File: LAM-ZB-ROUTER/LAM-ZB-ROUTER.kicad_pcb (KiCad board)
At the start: 2 copper layers, 40 x 60 mm, 12 parts, among them J1 PWR, J2 Conn_01x07_Pin, U1 CC2538, U2 LT1117-3.3

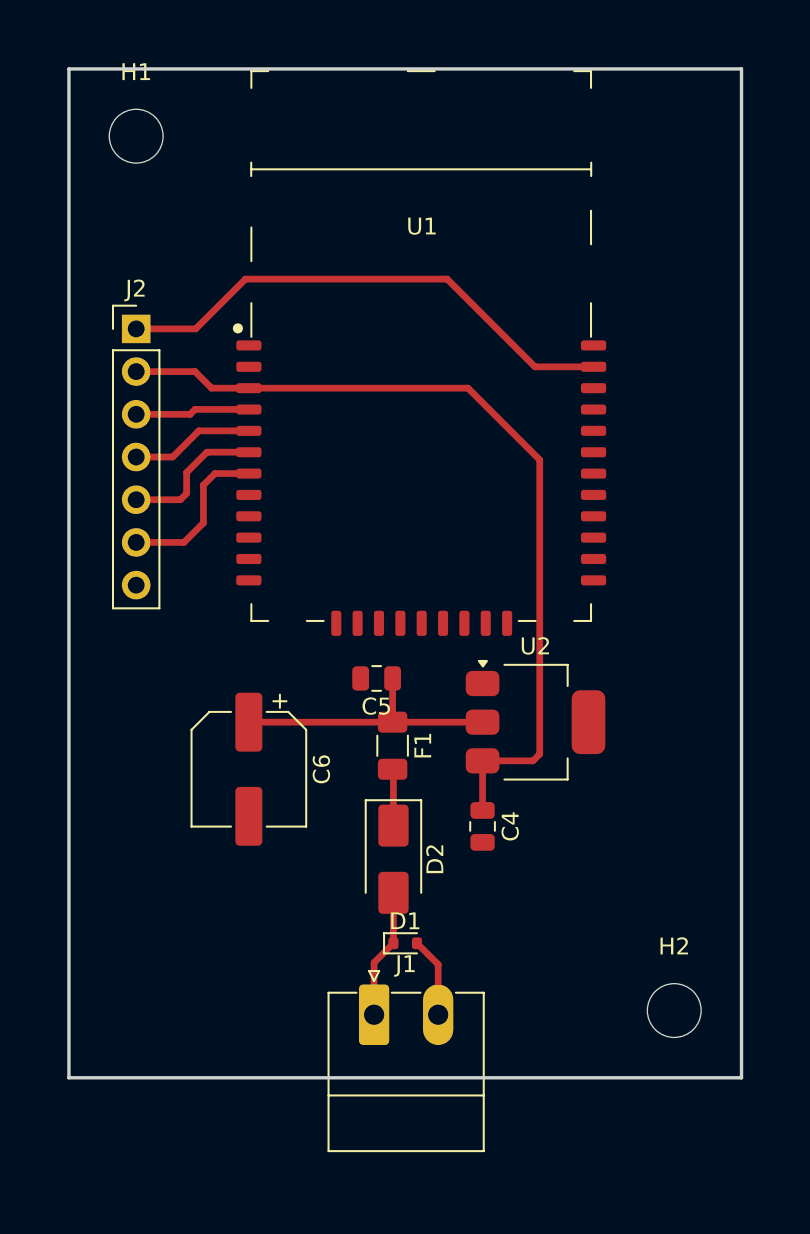
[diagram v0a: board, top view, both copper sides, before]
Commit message: LAM-ZB-ROUTER: Rev B
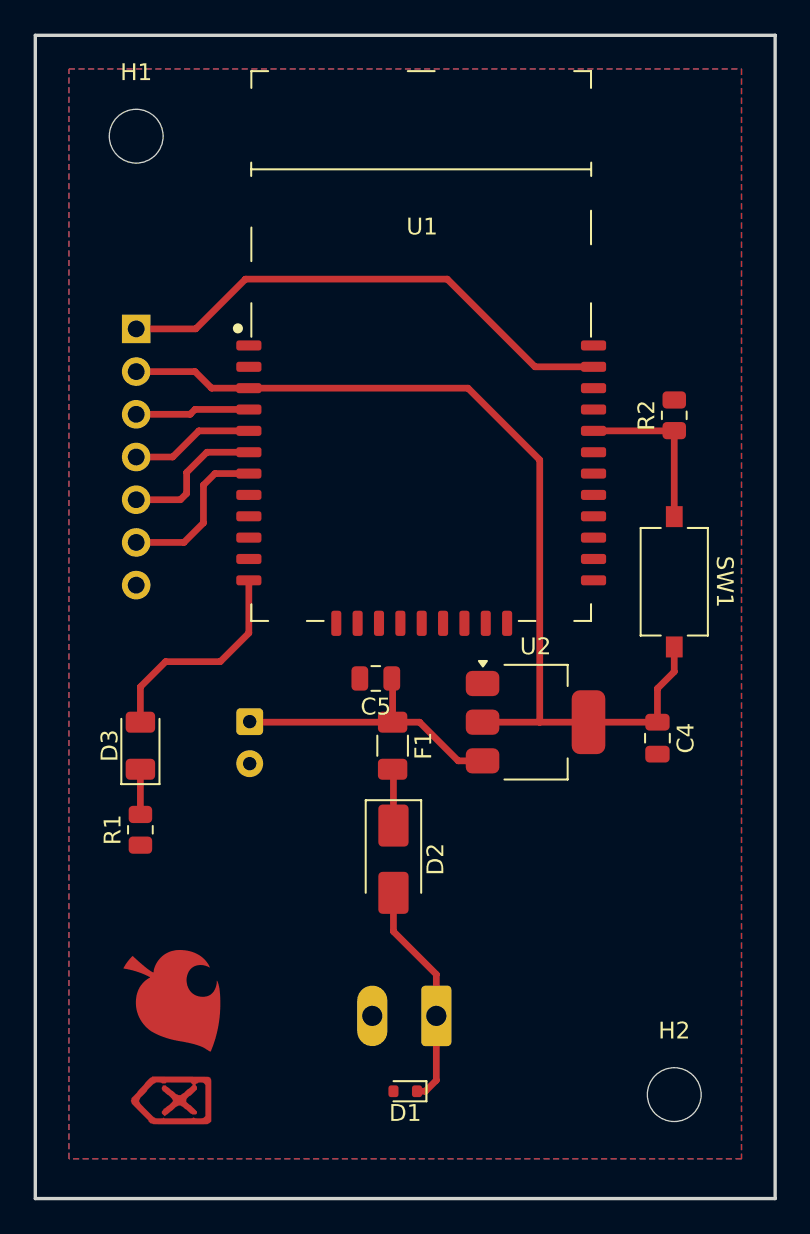
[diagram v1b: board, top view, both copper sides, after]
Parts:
- removed C6: 470uF / 25V, Capacitor_SMD:CP_Elec_6.3x5.9
- added C1: 100uF / 25V, Capacitor_THT:CP_Radial_D6.3mm_P2.50mm, B.Cu at (140.8, 108.8)
- added D3: RUN, LED_SMD:LED_1206_3216Metric, F.Cu at (134.2, 110.2)
- added R1: 270R, Resistor_SMD:R_0805_2012Metric, F.Cu at (134.2, 115.2)
- added R2: 5K1, Resistor_SMD:R_0805_2012Metric, F.Cu at (166.0, 90.6)
- added REF**: 0x08_F_Cu, Logos:0x08_F_Cu, F.Cu at (136.1, 131.3)
- added SW1: FLASH, Button_Switch_SMD:SW_Tactile_SPST_NO_Straight_CK_PTS636Sx25SMTRLFS, F.Cu at (166.0, 100.5)
- J1, J2: moved to B.Cu
- moved C4 11.7 mm to (165.0, 109.8)
- moved D1 8.80 mm to (150.0, 130.8), turned to 180 degrees
- moved H2 5.00 mm to (166.0, 131.0)
- moved J1 3.70 mm to (151.8, 126.3), turned to 180 degrees
- moved C5 0.05 mm to (148.2, 106.2)
- turned J2 to 180 degrees
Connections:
- U1 pad 12: unconnected-(U1-PB1-Pad12) -> Net-(D3-A)
- U1 pad 29: unconnected-(U1-PA7-Pad29) -> Net-(U1-PA7)
- U2 pad 2: +12V -> +3V3
- U2 pad 3: +3V3 -> +12V
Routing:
- net Net-(D3-A): track 0.00 -> 13.0 mm
- net Net-(U1-PA7): track 0.00 -> 9.92 mm
- net +3V3: track 50.2 -> 57.1 mm
- net Net-(D1-K): track 7.73 -> 13.6 mm
- net GND: track 4.77 -> 0.00 mm
- net Net-(D3-K): track 0.00 -> 2.69 mm
- net +12V: track 16.5 -> 17.5 mm
- added copper zone on B.Cu, net GND
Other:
- board size 40 x 60 mm -> 44 x 69.2 mm
